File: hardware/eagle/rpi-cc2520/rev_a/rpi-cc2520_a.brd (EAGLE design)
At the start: 30.5 x 39.5 mm, 21 parts, among them J1 PINHD-2X12/SMD, J2 PINHD-2X12/SMD, U1 CC2520

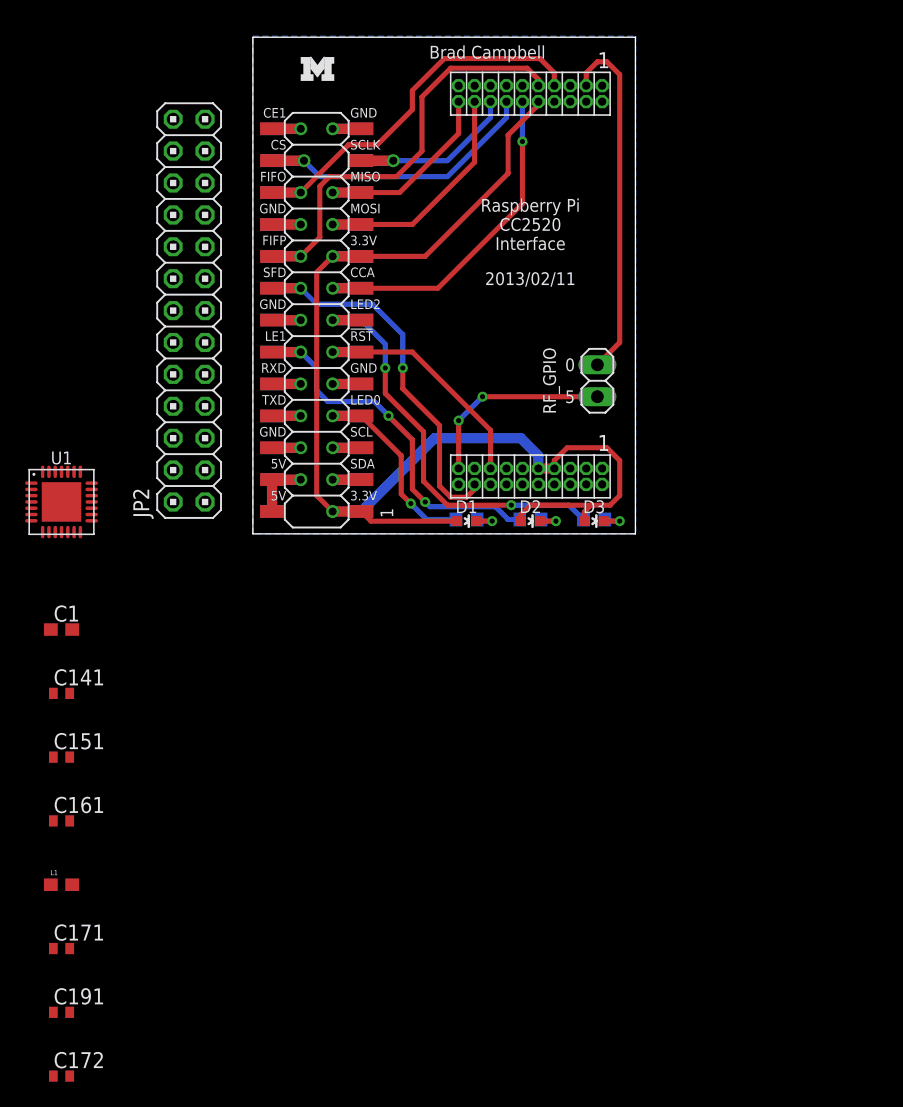
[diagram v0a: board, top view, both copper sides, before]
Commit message: laying out board
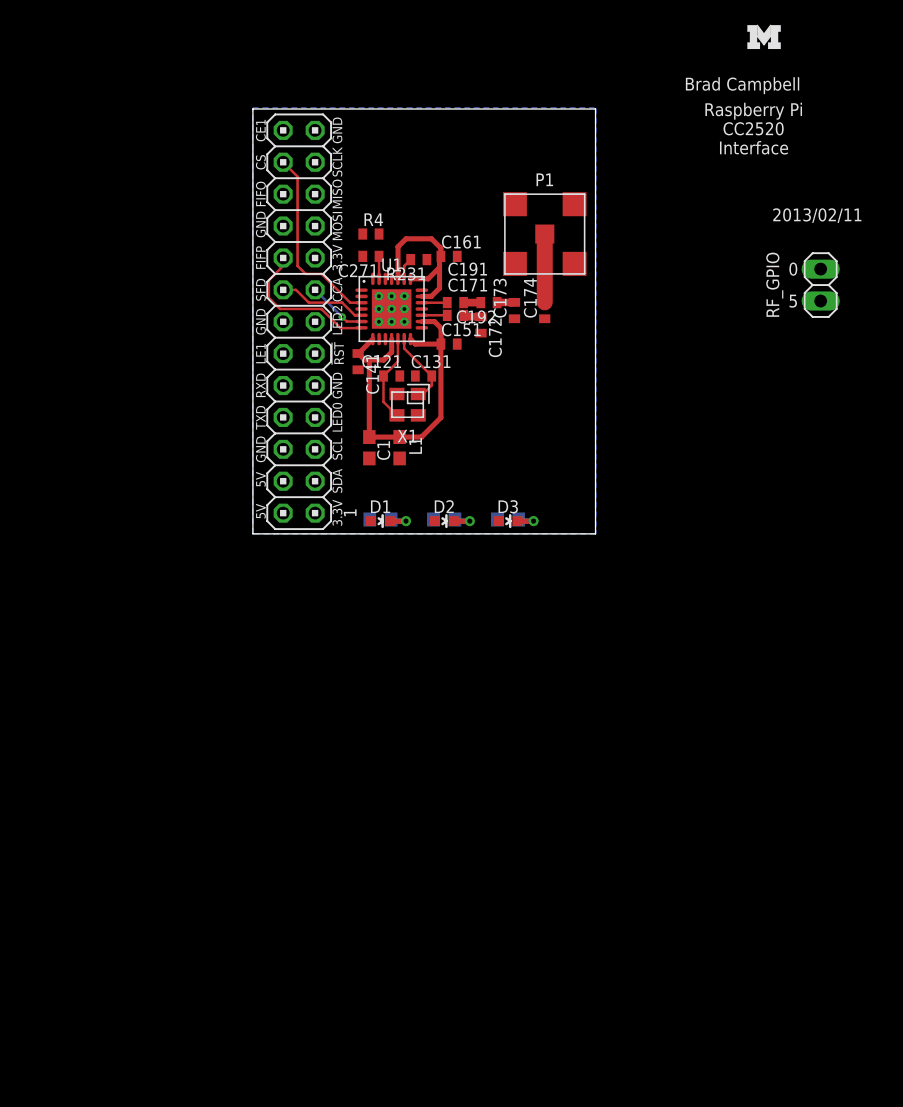
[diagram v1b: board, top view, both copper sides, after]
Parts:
- removed EVM1: CC2520EM, brouter:TI_CC_EVM
- removed J1, J2: PINHD-2X12/SMD, headers:2X13/SMD
- added C121, C131: 27pF, rcl:C0402
- added C173: 1.8pF, rcl:C0402
- added C174: 1pF, rcl:C0402
- added C192: 1.5pF, rcl:C0402
- added C271: 100nF, rcl:C0402
- added P1: MOLEX_73251-135X, connector:SMA-J/PCB
- added R231: 56k 1%, rcl:R0402
- added R4: 1M 1%, rcl:R0402
- added X1: NX2520SA, rpi-cc2520:NX2520SA
- moved C172 68.5 mm to (18.2, 16.6), turned to 270 degrees
- moved C191 64.6 mm to (16.1, 18.4), turned to 180 degrees
- moved C171 59.4 mm to (16.1, 17.4)
- moved C161 54.5 mm to (15.6, 22.1)
- moved C151 45.1 mm to (15.6, 15.1)
- moved L1 44.0 mm to (11.7, 6.86), turned to 270 degrees
- moved U$1 35.7 mm to (39.4, 38.6)
- moved C141 35.4 mm to (8.38, 13.7), turned to 270 degrees
- moved U1 30.5 mm to (11.0, 17.9)
- moved C1 28.5 mm to (9.27, 6.86), turned to 270 degrees
- moved JP1 19.3 mm to (45.2, 19.8)
- moved JP2 8.81 mm to (3.68, 16.9)
- moved D1 6.86 mm to (10.2, 1.02)
- moved D3 6.86 mm to (20.3, 1.02)
- moved R1 6.86 mm to (10.2, 1.14)
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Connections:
- new net N$10: C174.2, P1.1
- new net N$11: C131.1, U1.13, X1.1
- new net N$12: C271.1, U1.27
- new net N$13: C121.1, U1.12, X1.3
- new net N$14: R231.2, U1.23
- new net N$8: C191.1, C192.2
- new net N$9: C173.2, C192.1
- net !RESET: no longer EVM1.P2_15, J1.12, J2.11
- net 5V: no longer J1.1, J1.3, J2.2, J2.4
- net CCA: no longer EVM1.P1_12, J1.16, J2.15
- net CC_GPIO0: no longer EVM1.P1_3
- net CC_GPIO5: no longer EVM1.P2_19
- net CE0: no longer EVM1.P1_14, J1.23, J2.24
- net CE1: no longer J1.25, J2.26
- net FIFO: no longer EVM1.P1_7, J1.21, J2.22
- net FIFOP: no longer EVM1.P1_9, J1.17, J2.18
- net GND: now also C121.2, C131.2, C172.2, C173.1, C174.1, C271.2, P1.2, P1.3, P1.4, P1.5, R231.1, R4.1; no longer EVM1.P1_1, EVM1.P1_19, J1.10, J1.13, J1.19, J1.26, J1.5, J2.14, J2.20, J2.25, J2.6, J2.9
- net LED0: no longer J1.8, J2.7
- net LED1: no longer J1.11, J2.12
- net LED2: no longer J1.14, J2.13
- net MISO: now also R4.2; no longer EVM1.P1_20, J1.22, J2.21
- net MOSI: no longer EVM1.P1_18, J1.20, J2.19
- net SCL: no longer J1.6, J2.5
- net SCLK: no longer EVM1.P1_16, J1.24, J2.23
- net SDA: no longer J1.4, J2.3
- net SFD: no longer EVM1.P2_18, J1.15, J2.16
- net UART0_RXD: no longer J1.9, J2.10
- net UART0_TXD: no longer J1.7, J2.8
- net VCC: no longer EVM1.P1_10, EVM1.P2_7, EVM1.P2_9, J1.18, J1.2, J2.1, J2.17
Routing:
- net VCC: track 98.9 -> 0.00 mm, vias 2 -> 0
- net N$5: track 0.00 -> 43.9 mm
- net LED2: track 33.4 -> 0.00 mm, vias 3 -> 0
- net FIFO: track 31.6 -> 0.00 mm, vias 1 -> 0
- net LED1: track 30.9 -> 0.00 mm, vias 3 -> 0
- net CC_GPIO0: track 28.3 -> 0.00 mm
- net SFD: track 31.3 -> 7.08 mm, vias 2 -> 0
- net CCA: track 28.3 -> 4.74 mm, vias 2 -> 1
- net FIFOP: track 35.5 -> 12.0 mm, vias 1 -> 0
- net GND: track 22.9 -> 0.00 mm, vias 5 -> 9
- net !RESET: track 20.5 -> 0.00 mm, vias 1 -> 0
- net MOSI: track 20.5 -> 0.00 mm, vias 1 -> 0
- net LED0: track 17.3 -> 0.00 mm, vias 2 -> 0
- net MISO: track 16.8 -> 0.00 mm, vias 1 -> 0
- net CC_GPIO5: track 15.6 -> 0.00 mm, vias 2 -> 0
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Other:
- board size 30.5 x 39.5 mm -> 27.3 x 33.8 mm
